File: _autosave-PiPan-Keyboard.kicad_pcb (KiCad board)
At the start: 2 copper layers, 93 parts, among them J0 Conn_01x18_MountingPin, SW0 RotaryEncoder_Switch, U1 Pico

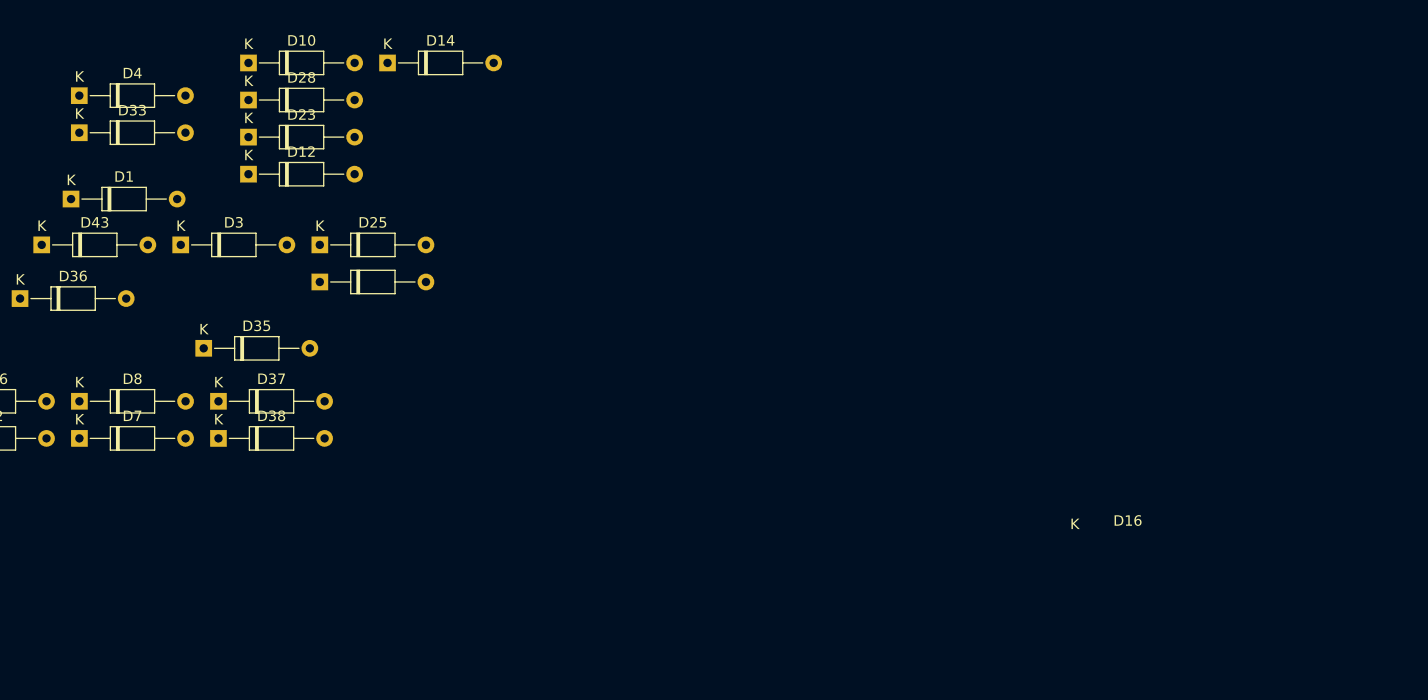
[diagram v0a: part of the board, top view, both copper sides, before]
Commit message: updated definitions
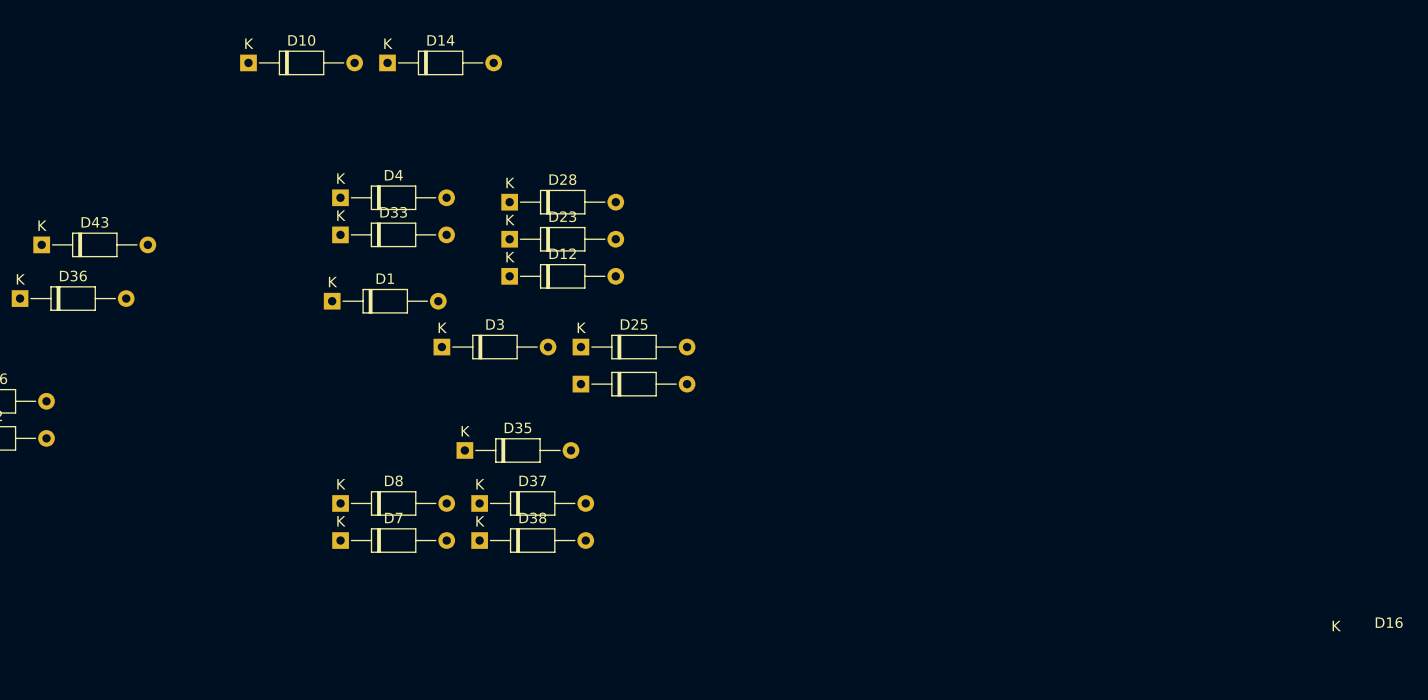
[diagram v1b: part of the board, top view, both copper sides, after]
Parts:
- moved D1 26.8 mm to (289.8, 165.4)
- moved D12 26.8 mm to (306.8, 163.0)
- moved D16 26.8 mm to (313.6, 173.3)
- moved D25 26.8 mm to (313.6, 169.7)
- moved D28 26.8 mm to (306.8, 155.9)
- moved D3 26.8 mm to (300.3, 169.7)
- moved D33 26.8 mm to (290.6, 159.0)
- moved D7 26.8 mm to (290.6, 188.3)
- moved D8 26.8 mm to (290.6, 184.7)
- moved D23 26.8 mm to (306.8, 159.4)
- moved D35 26.8 mm to (302.5, 179.6)
- moved D4 26.8 mm to (290.6, 155.5)
- moved D37 26.8 mm to (303.9, 184.7)
- moved D38 26.8 mm to (303.9, 188.3)
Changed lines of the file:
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@@
   )
   (footprint "Diode_THT:D_DO-35_SOD27_P10.16mm_Horizontal" (layer "F.Cu")
-    (at 265.5975 178.48375)
+    (at 290.595 188.26125)
     (descr "Diode, DO-35_SOD27 series, Axial, Horizontal, pin pitch=10.16mm, , length*diameter=4*2mm^2, , http://www.diodes.com/_files/packages/DO-35.pdf")
     (tags "Diode DO-35_SOD27 series Axial Horizontal pin pitch 10.16mm  length 4mm diameter 2mm")
@@
   )
   (footprint "Diode_THT:D_DO-35_SOD27_P10.16mm_Horizontal" (layer "F.Cu")
-    (at 288.6075 159.9625)
+    (at 313.605 169.74)
     (descr "Diode, DO-35_SOD27 series, Axial, Horizontal, pin pitch=10.16mm, , length*diameter=4*2mm^2, , http://www.diodes.com/_files/packages/DO-35.pdf")
     (tags "Diode DO-35_SOD27 series Axial Horizontal pin pitch 10.16mm  length 4mm diameter 2mm")
@@
   )
   (footprint "Diode_THT:D_DO-35_SOD27_P10.16mm_Horizontal" (layer "F.Cu")
-    (at 265.58875 145.675)
+    (at 290.58625 155.4525)
     (descr "Diode, DO-35_SOD27 series, Axial, Horizontal, pin pitch=10.16mm, , length*diameter=4*2mm^2, , http://www.diodes.com/_files/packages/DO-35.pdf")
     (tags "Diode DO-35_SOD27 series Axial Horizontal pin pitch 10.16mm  length 4mm diameter 2mm")
@@
   )
   (footprint "Diode_THT:D_DO-35_SOD27_P10.16mm_Horizontal" (layer "F.Cu")
-    (at 277.495 169.8625)
+    (at 302.4925 179.64)
     (descr "Diode, DO-35_SOD27 series, Axial, Horizontal, pin pitch=10.16mm, , length*diameter=4*2mm^2, , http://www.diodes.com/_files/packages/DO-35.pdf")
     (tags "Diode DO-35_SOD27 series Axial Horizontal pin pitch 10.16mm  length 4mm diameter 2mm")
@@
   )
   (footprint "Diode_THT:D_DO-35_SOD27_P10.16mm_Horizontal" (layer "F.Cu")
-    (at 278.9075 174.93375)
+    (at 303.905 184.71125)
     (descr "Diode, DO-35_SOD27 series, Axial, Horizontal, pin pitch=10.16mm, , length*diameter=4*2mm^2, , http://www.diodes.com/_files/packages/DO-35.pdf")
     (tags "Diode DO-35_SOD27 series Axial Horizontal pin pitch 10.16mm  length 4mm diameter 2mm")
@@
   )
   (footprint "Diode_THT:D_DO-35_SOD27_P10.16mm_Horizontal" (layer "F.Cu")
-    (at 278.9075 178.48375)
+    (at 303.905 188.26125)
     (descr "Diode, DO-35_SOD27 series, Axial, Horizontal, pin pitch=10.16mm, , length*diameter=4*2mm^2, , http://www.diodes.com/_files/packages/DO-35.pdf")
     (tags "Diode DO-35_SOD27 series Axial Horizontal pin pitch 10.16mm  length 4mm diameter 2mm")
@@
       (effects (font (size 1 1) (thickness 0.15)))
     )
-    (fp_text value "D_Small" (at 16.4775 33.50375) (layer "F.Fab")
+    (fp_text value "D_Small" (at 41.475 43.28125) (layer "F.Fab")
       (effects (font (size 1 1) (thickness 0.15)))
     )
@@
   )
   (footprint "Diode_THT:D_DO-35_SOD27_P10.16mm_Horizontal" (layer "F.Cu")
-    (at 281.78125 153.19375)
+    (at 306.77875 162.97125)
     (descr "Diode, DO-35_SOD27 series, Axial, Horizontal, pin pitch=10.16mm, , length*diameter=4*2mm^2, , http://www.diodes.com/_files/packages/DO-35.pdf")
     (tags "Diode DO-35_SOD27 series Axial Horizontal pin pitch 10.16mm  length 4mm diameter 2mm")
@@
   )
   (footprint "Diode_THT:D_DO-35_SOD27_P10.16mm_Horizontal" (layer "F.Cu")
-    (at 264.795 155.575)
+    (at 289.7925 165.3525)
     (descr "Diode, DO-35_SOD27 series, Axial, Horizontal, pin pitch=10.16mm, , length*diameter=4*2mm^2, , http://www.diodes.com/_files/packages/DO-35.pdf")
     (tags "Diode DO-35_SOD27 series Axial Horizontal pin pitch 10.16mm  length 4mm diameter 2mm")
@@
   )
   (footprint "Diode_THT:D_DO-35_SOD27_P10.16mm_Horizontal" (layer "F.Cu")
-    (at 281.78125 146.09375)
+    (at 306.77875 155.87125)
     (descr "Diode, DO-35_SOD27 series, Axial, Horizontal, pin pitch=10.16mm, , length*diameter=4*2mm^2, , http://www.diodes.com/_files/packages/DO-35.pdf")
     (tags "Diode DO-35_SOD27 series Axial Horizontal pin pitch 10.16mm  length 4mm diameter 2mm")
@@
   )
   (footprint "Diode_THT:D_DO-35_SOD27_P10.16mm_Horizontal" (layer "F.Cu")
-    (at 281.78125 149.64375)
+    (at 306.77875 159.42125)
     (descr "Diode, DO-35_SOD27 series, Axial, Horizontal, pin pitch=10.16mm, , length*diameter=4*2mm^2, , http://www.diodes.com/_files/packages/DO-35.pdf")
     (tags "Diode DO-35_SOD27 series Axial Horizontal pin pitch 10.16mm  length 4mm diameter 2mm")
@@
   )
   (footprint "Diode_THT:D_DO-35_SOD27_P10.16mm_Horizontal" (layer "F.Cu")
-    (at 275.2975 159.9625)
+    (at 300.295 169.74)
     (descr "Diode, DO-35_SOD27 series, Axial, Horizontal, pin pitch=10.16mm, , length*diameter=4*2mm^2, , http://www.diodes.com/_files/packages/DO-35.pdf")
     (tags "Diode DO-35_SOD27 series Axial Horizontal pin pitch 10.16mm  length 4mm diameter 2mm")
@@
   )
   (footprint "Diode_THT:D_DO-35_SOD27_P10.16mm_Horizontal" (layer "F.Cu")
-    (at 288.6075 163.5125)
+    (at 313.605 173.29)
     (descr "Diode, DO-35_SOD27 series, Axial, Horizontal, pin pitch=10.16mm, , length*diameter=4*2mm^2, , http://www.diodes.com/_files/packages/DO-35.pdf")
     (tags "Diode DO-35_SOD27 series Axial Horizontal pin pitch 10.16mm  length 4mm diameter 2mm")
@@
       (effects (font (size 1 1) (thickness 0.15)))
     )
-    (fp_text value "D_Small" (at 77.34625 27.11) (layer "F.Fab")
+    (fp_text value "D_Small" (at 102.34375 36.8875) (layer "F.Fab")
       (effects (font (size 1 1) (thickness 0.15)))
     )
@@
   )
   (footprint "Diode_THT:D_DO-35_SOD27_P10.16mm_Horizontal" (layer "F.Cu")
-    (at 265.5975 174.93375)
+    (at 290.595 184.71125)
     (descr "Diode, DO-35_SOD27 series, Axial, Horizontal, pin pitch=10.16mm, , length*diameter=4*2mm^2, , http://www.diodes.com/_files/packages/DO-35.pdf")
     (tags "Diode DO-35_SOD27 series Axial Horizontal pin pitch 10.16mm  length 4mm diameter 2mm")
@@
   )
   (footprint "Diode_THT:D_DO-35_SOD27_P10.16mm_Horizontal" (layer "F.Cu")
-    (at 265.58875 149.225)
+    (at 290.58625 159.0025)
     (descr "Diode, DO-35_SOD27 series, Axial, Horizontal, pin pitch=10.16mm, , length*diameter=4*2mm^2, , http://www.diodes.com/_files/packages/DO-35.pdf")
     (tags "Diode DO-35_SOD27 series Axial Horizontal pin pitch 10.16mm  length 4mm diameter 2mm")
